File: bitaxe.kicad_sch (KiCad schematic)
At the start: 92 parts, among them IC1 BM1387, IC2 BM1387, IC3 MIC5317, IC4 MIC5317, J2 Conn_01x02, J3 Conn_01x05, J4 Conn_01x02, J5 Conn_01x03, Y1 25MHz

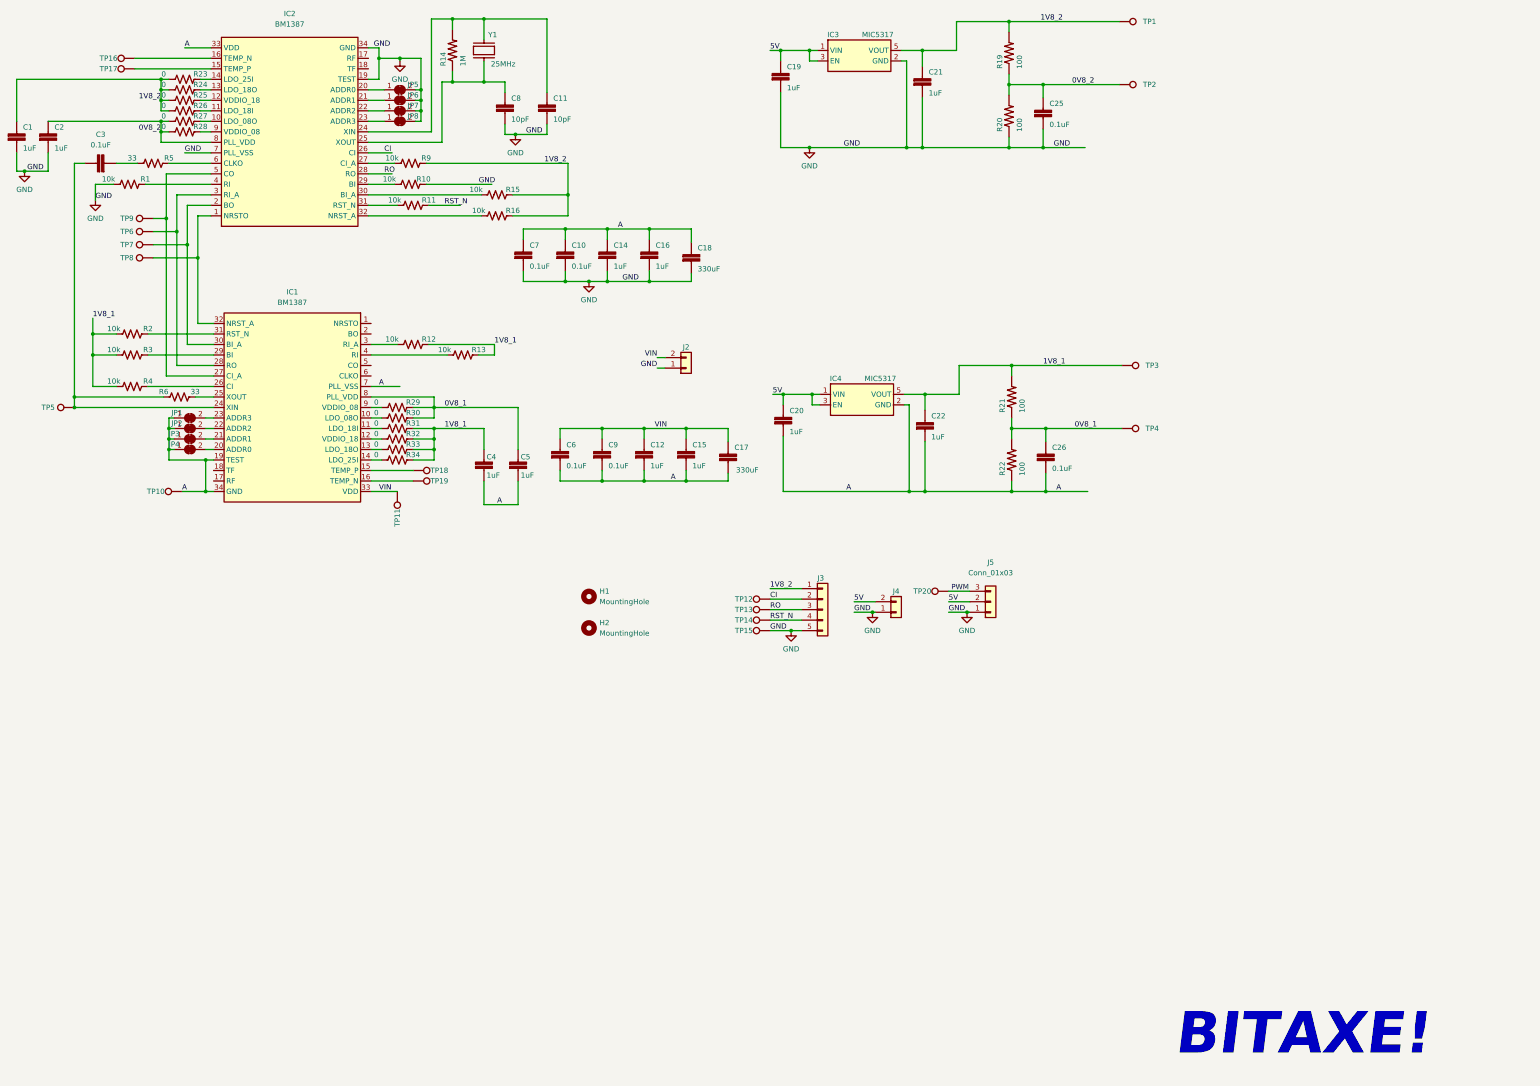
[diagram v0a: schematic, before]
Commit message: schematic cleanup
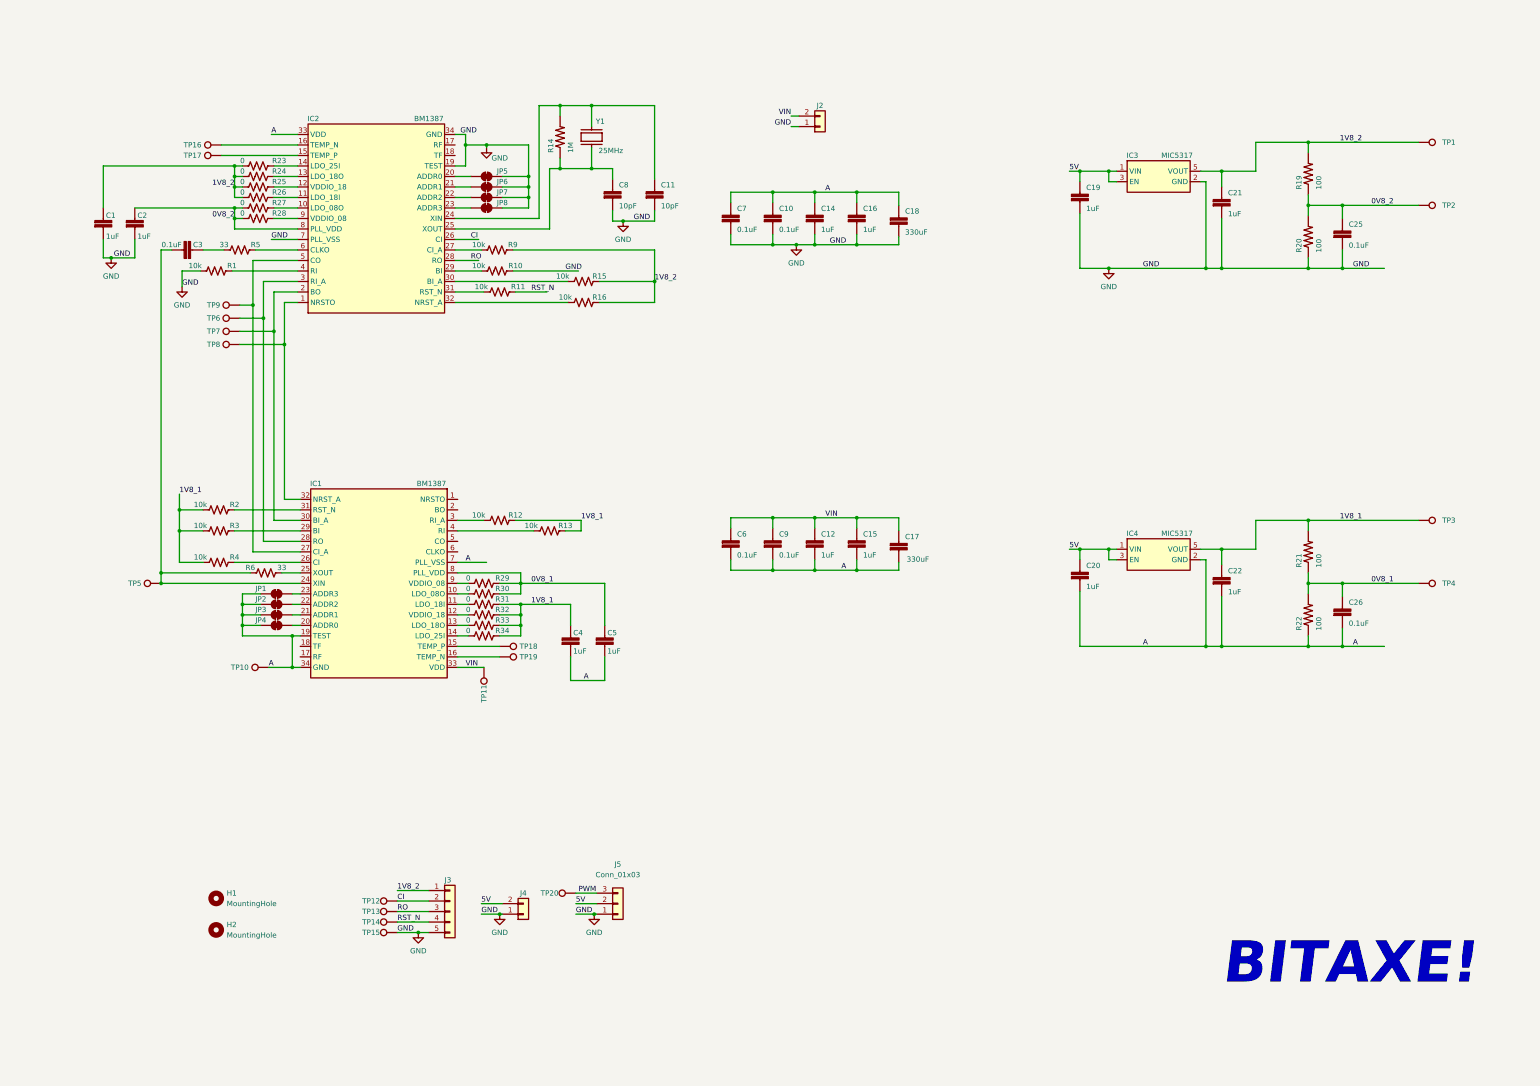
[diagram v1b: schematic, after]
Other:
- moved on the sheet: C1, C10, C11, C12, C14, C15, C16, C17, C18, C19, C2, C20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
